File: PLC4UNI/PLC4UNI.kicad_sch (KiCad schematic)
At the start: 0 parts

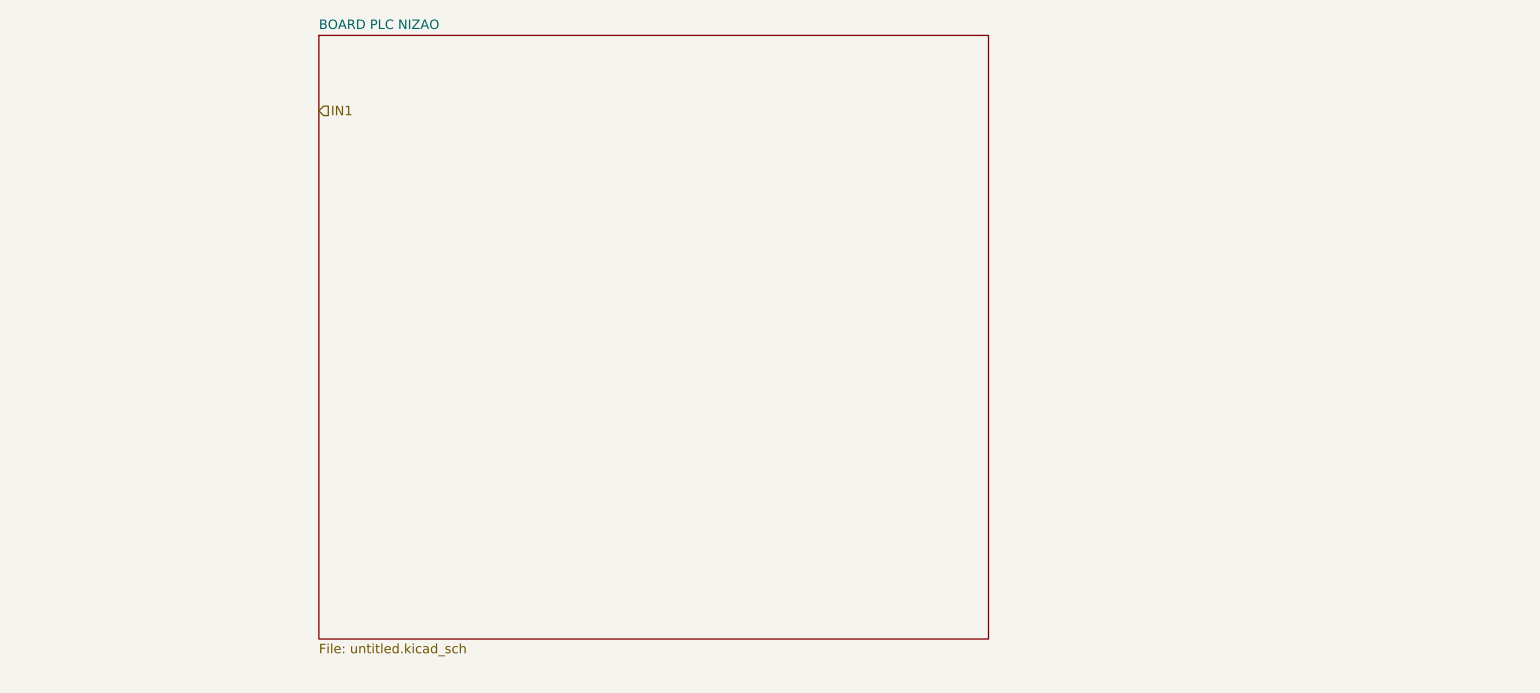
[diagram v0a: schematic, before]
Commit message: esquematico general, sin circuitos definidos
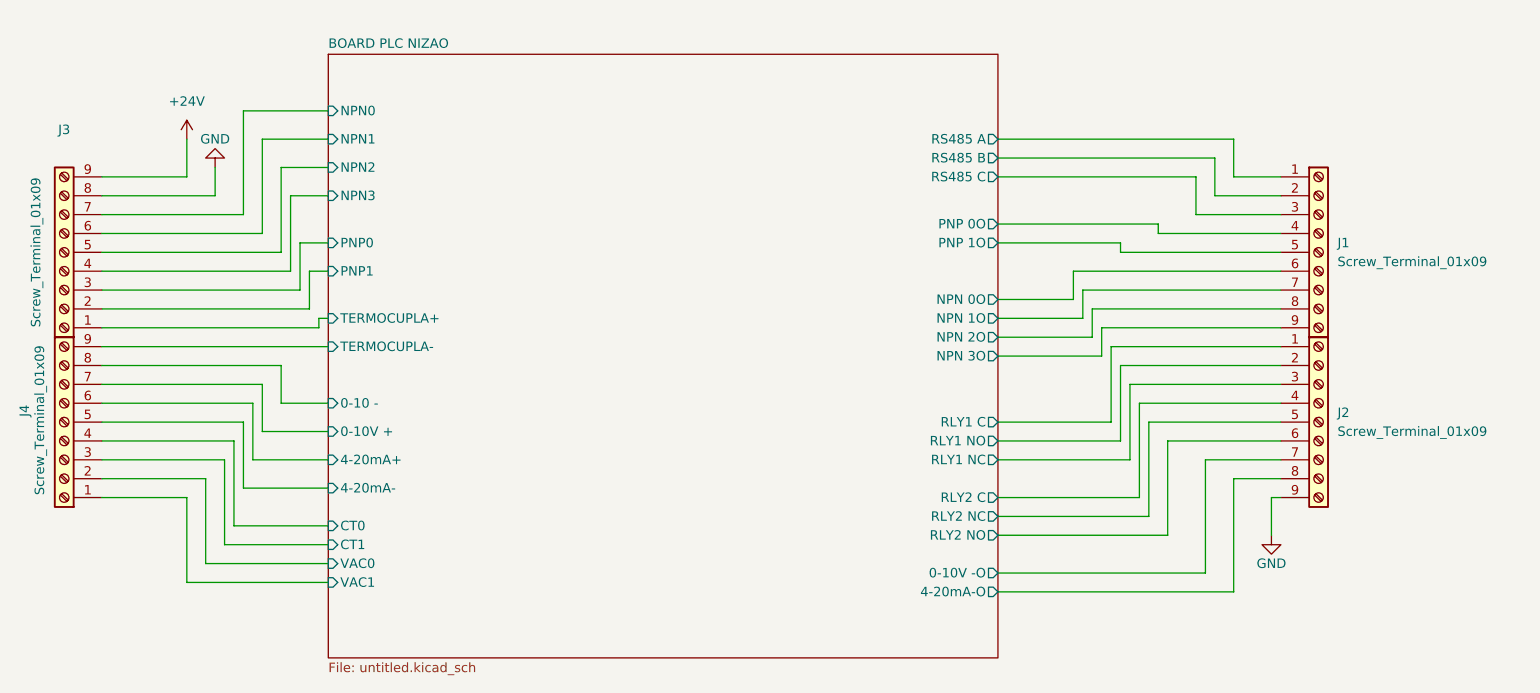
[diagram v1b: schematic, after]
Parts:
- added J1, J2, J3, J4: Screw_Terminal_01x09, symbol Connector:Screw_Terminal_01x09
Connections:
- new net +24V: J3.9 (Pin_9)
- new net BOARD PLC NIZAO/0-10 -: J4.8 (Pin_8)
- new net BOARD PLC NIZAO/0-10V +: J4.7 (Pin_7)
- new net BOARD PLC NIZAO/0-10V -O: J2.7 (Pin_7)
- new net BOARD PLC NIZAO/4-20mA+: J4.6 (Pin_6)
- new net BOARD PLC NIZAO/4-20mA-: J4.5 (Pin_5)
- new net BOARD PLC NIZAO/4-20mA-O: J2.8 (Pin_8)
- new net BOARD PLC NIZAO/CT0: J4.4 (Pin_4)
- new net BOARD PLC NIZAO/CT1: J4.3 (Pin_3)
- new net BOARD PLC NIZAO/NPN 0O: J1.6 (Pin_6)
- new net BOARD PLC NIZAO/NPN 1O: J1.7 (Pin_7)
- new net BOARD PLC NIZAO/NPN 2O: J1.8 (Pin_8)
- new net BOARD PLC NIZAO/NPN 3O: J1.9 (Pin_9)
- new net BOARD PLC NIZAO/NPN0: J3.7 (Pin_7)
- new net BOARD PLC NIZAO/NPN1: J3.6 (Pin_6)
- new net BOARD PLC NIZAO/NPN2: J3.5 (Pin_5)
- new net BOARD PLC NIZAO/NPN3: J3.4 (Pin_4)
- new net BOARD PLC NIZAO/PNP 0O: J1.4 (Pin_4)
- new net BOARD PLC NIZAO/PNP 1O: J1.5 (Pin_5)
- new net BOARD PLC NIZAO/PNP0: J3.3 (Pin_3)
- new net BOARD PLC NIZAO/PNP1: J3.2 (Pin_2)
- new net BOARD PLC NIZAO/RLY1 C: J2.1 (Pin_1)
- new net BOARD PLC NIZAO/RLY1 NC: J2.3 (Pin_3)
- new net BOARD PLC NIZAO/RLY1 NO: J2.2 (Pin_2)
- new net BOARD PLC NIZAO/RLY2 C: J2.4 (Pin_4)
- new net BOARD PLC NIZAO/RLY2 NC: J2.5 (Pin_5)
- new net BOARD PLC NIZAO/RLY2 NO: J2.6 (Pin_6)
- new net BOARD PLC NIZAO/RS485 A: J1.1 (Pin_1)
- new net BOARD PLC NIZAO/RS485 B: J1.2 (Pin_2)
- new net BOARD PLC NIZAO/RS485 C: J1.3 (Pin_3)
- new net BOARD PLC NIZAO/TERMOCUPLA+: J3.1 (Pin_1)
- new net BOARD PLC NIZAO/TERMOCUPLA-: J4.9 (Pin_9)
- new net BOARD PLC NIZAO/VAC0: J4.2 (Pin_2)
- new net BOARD PLC NIZAO/VAC1: J4.1 (Pin_1)
- new net GND: J2.9 (Pin_9), J3.8 (Pin_8)
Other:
- sheet BOARD PLC NIZAO ports: added 0-10 -, 0-10V +, 0-10V -O, 4-20mA+, 4-20mA-, 4-20mA-O, CT0, CT1, NPN 0O, NPN 1O, NPN 2O, NPN 3O, NPN0, NPN1, NPN2, NPN3, PNP 0O, PNP 1O, PNP0, PNP1, RLY1 C, RLY1 NC, RLY1 NO, RLY2 C, RLY2 NC, RLY2 NO, RS485 A, RS485 B, RS485 C, TERMOCUPLA+, TERMOCUPLA-, VAC0, VAC1; removed none
